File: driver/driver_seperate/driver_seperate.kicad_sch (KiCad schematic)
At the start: 2 parts, among them J1 Conn_01x03, J3 Conn_01x07

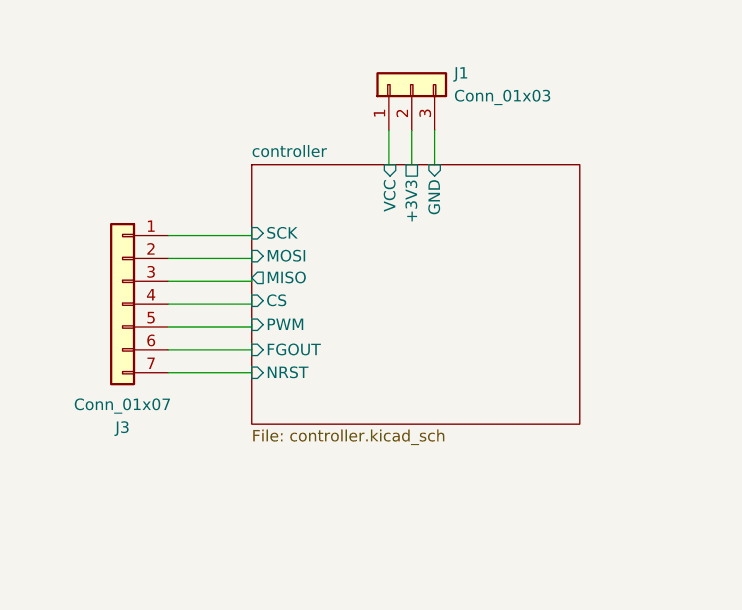
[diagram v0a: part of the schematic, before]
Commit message: Add start of new design
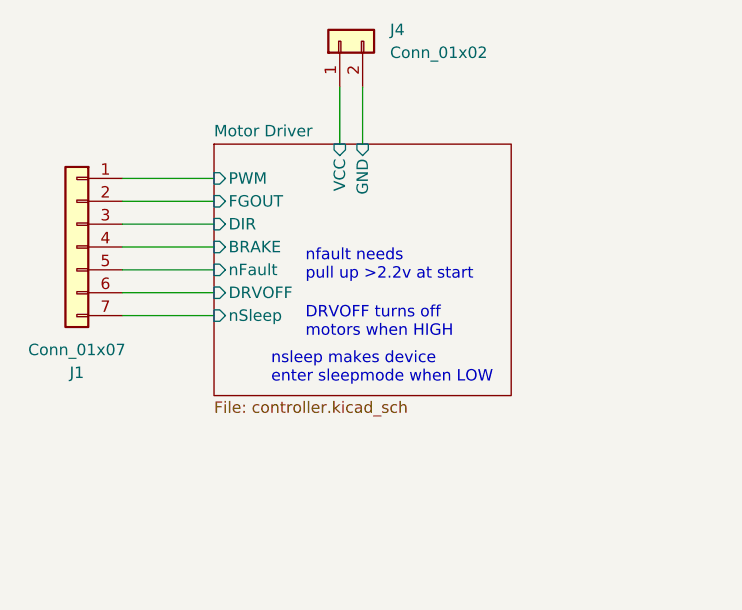
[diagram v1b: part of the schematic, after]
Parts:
- removed J1: Conn_01x03, Connector_Molex:Molex_CLIK-Mate_502443-0370_1x03-1MP_P2.00mm_Vertical, symbol Connector_Generic:Conn_01x03
- removed J3: Conn_01x07, Connector_Molex:Molex_CLIK-Mate_502382-0770_1x07-1MP_P1.25mm_Vertical, symbol Connector_Generic:Conn_01x07
- added J1: Conn_01x07, Connector_Molex:Molex_KK-254_AE-6410-07A_1x07_P2.54mm_Vertical, symbol Connector_Generic:Conn_01x07
- added J4: Conn_01x02, Connector_Molex:Molex_KK-254_AE-6410-02A_1x02_P2.54mm_Vertical, symbol Connector_Generic:Conn_01x02
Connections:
- net Motor Driver/FGOUT: now also J1.2 (Pin_2)
- net Motor Driver/GND: now also J4.2 (Pin_2)
- net Motor Driver/PWM: now also J1.1 (Pin_1)
- net Motor Driver/VCC: now also J4.1 (Pin_1)
- new net Motor Driver/BRAKE: J1.4 (Pin_4)
- new net Motor Driver/DIR: J1.3 (Pin_3)
- new net Motor Driver/DRVOFF: J1.6 (Pin_6)
- new net Motor Driver/nFault: J1.5 (Pin_5)
- new net Motor Driver/nSleep: J1.7 (Pin_7)
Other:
- sheet controller renamed Motor Driver
- sheet Motor Driver ports: added BRAKE, DIR, DRVOFF, nFault, nSleep; removed +3V3, CS, MISO, MOSI, NRST, SCK
- note added: "DRVOFF turns off motors when HIGH"
- note added: "nfault needs pull up >2.2v at start"
- note added: "nsleep makes device enter sleepmode when LOW"
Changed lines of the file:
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@@
 (kicad_sch (version 20230121) (generator eeschema)
   (paper "A4")
-  (wire (pts (xy 48.641 50.8) (xy 48.641 50.546))
+  (wire (pts (xy 60.96 24.13) (xy 60.96 30.48))
     (stroke (width 0) (type default))
   )
-  (wire (pts (xy 68.961 28.956) (xy 68.961 32.766))
+  (wire (pts (xy 34.29 36.83) (xy 44.45 36.83))
     (stroke (width 0) (type default))
   )
-  (wire (pts (xy 39.37 45.72) (xy 48.641 45.72))
+  (wire (pts (xy 34.29 34.29) (xy 44.45 34.29))
     (stroke (width 0) (type default))
   )
-  (wire (pts (xy 66.421 32.766) (xy 66.421 28.956))
+  (wire (pts (xy 34.29 49.53) (xy 44.45 49.53))
     (stroke (width 0) (type default))
   )
-  (wire (pts (xy 63.881 32.766) (xy 64.008 32.766))
+  (wire (pts (xy 58.42 24.13) (xy 58.42 30.48))
     (stroke (width 0) (type default))
   )
-  (wire (pts (xy 39.37 50.8) (xy 48.641 50.8))
+  (wire (pts (xy 34.29 39.37) (xy 44.45 39.37))
     (stroke (width 0) (type default))
   )
-  (wire (pts (xy 39.37 48.26) (xy 48.641 48.26))
+  (wire (pts (xy 34.29 44.45) (xy 44.45 44.45))
     (stroke (width 0) (type default))
   )
-  (wire (pts (xy 48.641 40.64) (xy 48.641 40.386))
+  (wire (pts (xy 34.29 46.99) (xy 44.45 46.99))
     (stroke (width 0) (type default))
   )
-  (wire (pts (xy 39.37 53.34) (xy 48.641 53.34))
+  (wire (pts (xy 34.29 41.91) (xy 44.45 41.91))
     (stroke (width 0) (type default))
   )
-  (wire (pts (xy 48.641 45.72) (xy 48.641 45.339))
-    (stroke (width 0) (type default))
+  (text "nfault needs\npull up >2.2v at start" (at 54.61 45.72 0)
+    (effects (font (size 1.27 1.27)) (justify left bottom))
   )
-  (wire (pts (xy 39.37 55.88) (xy 48.641 55.88))
-    (stroke (width 0) (type default))
+  (text "DRVOFF turns off \nmotors when HIGH" (at 54.61 52.07 0)
+    (effects (font (size 1.27 1.27)) (justify left bottom))
   )
-  (wire (pts (xy 39.37 43.18) (xy 48.641 43.18))
-    (stroke (width 0) (type default))
-  )
-  (wire (pts (xy 63.881 28.956) (xy 63.881 32.766))
-    (stroke (width 0) (type default))
-  )
-  (wire (pts (xy 39.37 40.64) (xy 48.641 40.64))
-    (stroke (width 0) (type default))
-  )
-  (wire (pts (xy 48.641 43.18) (xy 48.641 42.926))
-    (stroke (width 0) (type default))
-  )
-  (wire (pts (xy 48.641 48.26) (xy 48.641 47.879))
-    (stroke (width 0) (type default))
+  (text "nsleep makes device \nenter sleepmode when LOW" (at 50.8 57.15 0)
+    (effects (font (size 1.27 1.27)) (justify left bottom))
   )
   (text "2" (at 269.24 194.31 0)
     (effects (font (size 1.27 1.27)) (justify left bottom))
   )
-  (symbol (lib_id "Connector_Generic:Conn_01x07") (at 34.29 48.26 0) (mirror y) (unit 1)
+  (symbol (lib_id "Connector_Generic:Conn_01x07") (at 29.21 41.91 0) (mirror y) (unit 1)
     (in_bom yes) (on_board yes) (dnp no)
-    (property "Reference" "J3" (at 34.29 61.976 0)
+    (property "Reference" "J1" (at 29.21 55.88 0)
       (effects (font (size 1.27 1.27)))
     )
-    (property "Value" "Conn_01x07" (at 34.29 59.436 0)
+    (property "Value" "Conn_01x07" (at 29.21 53.34 0)
       (effects (font (size 1.27 1.27)))
     )
-    (property "Footprint" "Connector_Molex:Molex_CLIK-Mate_502382-0770_1x07-1MP_P1.25mm_Vertical" (at 34.29 48.26 0)
+    (property "Footprint" "Connector_Molex:Molex_KK-254_AE-6410-07A_1x07_P2.54mm_Vertical" (at 29.21 41.91 0)
       (effects (font (size 1.27 1.27)) hide)
     )
-    (property "Datasheet" "~" (at 34.29 48.26 0)
+    (property "Datasheet" "~" (at 29.21 41.91 0)
       (effects (font (size 1.27 1.27)) hide)
     )
+    (pin "1")
+    (pin "7")
     (pin "5")
-    (pin "1")
+    (pin "4")
+    (pin "3")
     (pin "2")
-    (pin "4")
     (pin "6")
-    (pin "3")
-    (pin "7")
-    (instances
-      (project "driver_seperate"
-        (path "/8aa936d6-33ab-4874-8145-d1c763a0b8a3"
-          (reference "J3") (unit 1)
-        )
-      )
-    )
-  )
-  (symbol (lib_id "Connector_Generic:Conn_01x03") (at 66.421 23.876 90) (unit 1)
-    (in_bom yes) (on_board yes) (dnp no) (fields_autoplaced)
-    (property "Reference" "J1" (at 71.12 22.606 90)
-      (effects (font (size 1.27 1.27)) (justify right))
-    )
-    (property "Value" "Conn_01x03" (at 71.12 25.146 90)
-      (effects (font (size 1.27 1.27)) (justify right))
-    )
-    (property "Footprint" "Connector_Molex:Molex_CLIK-Mate_502443-0370_1x03-1MP_P2.00mm_Vertical" (at 66.421 23.876 0)
-      (effects (font (size 1.27 1.27)) hide)
-    )
-    (property "Datasheet" "~" (at 66.421 23.876 0)
-      (effects (font (size 1.27 1.27)) hide)
-    )
-    (pin "3")
-    (pin "1")
-    (pin "2")
     (instances
       (project "driver_seperate"
@@
     )
   )
-  (sheet (at 48.641 32.766) (size 36.449 28.829) (fields_autoplaced)
+  (symbol (lib_id "Connector_Generic:Conn_01x02") (at 58.42 19.05 90) (unit 1)
+    (in_bom yes) (on_board yes) (dnp no) (fields_autoplaced)
+    (property "Reference" "J4" (at 64.008 17.78 90)
+      (effects (font (size 1.27 1.27)) (justify right))
+    )
+    (property "Value" "Conn_01x02" (at 64.008 20.32 90)
+      (effects (font (size 1.27 1.27)) (justify right))
+    )
+    (property "Footprint" "Connector_Molex:Molex_KK-254_AE-6410-02A_1x02_P2.54mm_Vertical" (at 58.42 19.05 0)
+      (effects (font (size 1.27 1.27)) hide)
+    )
+    (property "Datasheet" "~" (at 58.42 19.05 0)
+      (effects (font (size 1.27 1.27)) hide)
+    )
+    (pin "2")
+    (pin "1")
+    (instances
+      (project "driver_seperate"
+        (path "/8aa936d6-33ab-4874-8145-d1c763a0b8a3"
+          (reference "J4") (unit 1)
+        )
+      )
+    )
+  )
+  (sheet (at 44.45 30.48) (size 33.02 27.94) (fields_autoplaced)
     (stroke (width 0.1524) (type solid))
     (fill (color 0 0 0 0.0000))
-    (property "Sheetname" "controller" (at 48.641 32.0544 0)
+    (property "Sheetname" "Motor Driver" (at 44.45 29.7684 0)
       (effects (font (size 1.27 1.27)) (justify left bottom))
     )
-    (property "Sheetfile" "controller.kicad_sch" (at 48.641 62.1796 0)
+    (property "Sheetfile" "controller.kicad_sch" (at 44.45 59.0046 0)
       (effects (font (size 1.27 1.27)) (justify left top))
     )
-    (pin "GND" input (at 68.961 32.766 90)
+    (pin "FGOUT" input (at 44.45 36.83 180)
+      (effects (font (size 1.27 1.27)) (justify left))
+    )
+    (pin "DIR" input (at 44.45 39.37 180)
+      (effects (font (size 1.27 1.27)) (justify left))
+    )
+    (pin "PWM" input (at 44.45 34.29 180)
+      (effects (font (size 1.27 1.27)) (justify left))
+    )
+    (pin "nSleep" input (at 44.45 49.53 180)
+      (effects (font (size 1.27 1.27)) (justify left))
+    )
+    (pin "DRVOFF" input (at 44.45 46.99 180)
+      (effects (font (size 1.27 1.27)) (justify left))
+    )
+    (pin "nFault" input (at 44.45 44.45 180)
+      (effects (font (size 1.27 1.27)) (justify left))
+    )
+    (pin "BRAKE" input (at 44.45 41.91 180)
+      (effects (font (size 1.27 1.27)) (justify left))
+    )
+    (pin "VCC" input (at 58.42 30.48 90)
       (effects (font (size 1.27 1.27)) (justify right))
     )
-    (pin "VCC" input (at 64.008 32.766 90)
+    (pin "GND" input (at 60.96 30.48 90)
       (effects (font (size 1.27 1.27)) (justify right))
     )
-    (pin "PWM" input (at 48.641 50.546 180)
-      (effects (font (size 1.27 1.27)) (justify left))
-    )
-    (pin "FGOUT" input (at 48.641 53.34 180)
-      (effects (font (size 1.27 1.27)) (justify left))
-    )
-    (pin "+3V3" passive (at 66.421 32.766 90)
-      (effects (font (size 1.27 1.27)) (justify right))
-    )
-    (pin "NRST" input (at 48.641 55.88 180)
-      (effects (font (size 1.27 1.27)) (justify left))
-    )
-    (pin "CS" input (at 48.641 47.879 180)
-      (effects (font (size 1.27 1.27)) (justify left))
-    )
-    (pin "MOSI" input (at 48.641 42.926 180)
-      (effects (font (size 1.27 1.27)) (justify left))
-    )
-    (pin "MISO" output (at 48.641 45.339 180)
-      (effects (font (size 1.27 1.27)) (justify left))
-    )
-    (pin "SCK" input (at 48.641 40.386 180)
-      (effects (font (size 1.27 1.27)) (justify left))
-    )
     (instances
